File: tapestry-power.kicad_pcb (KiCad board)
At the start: 2 copper layers, 15 parts, among them J1 4.5-20V, J2 4.5-20V, J3 5V, U1 sic450

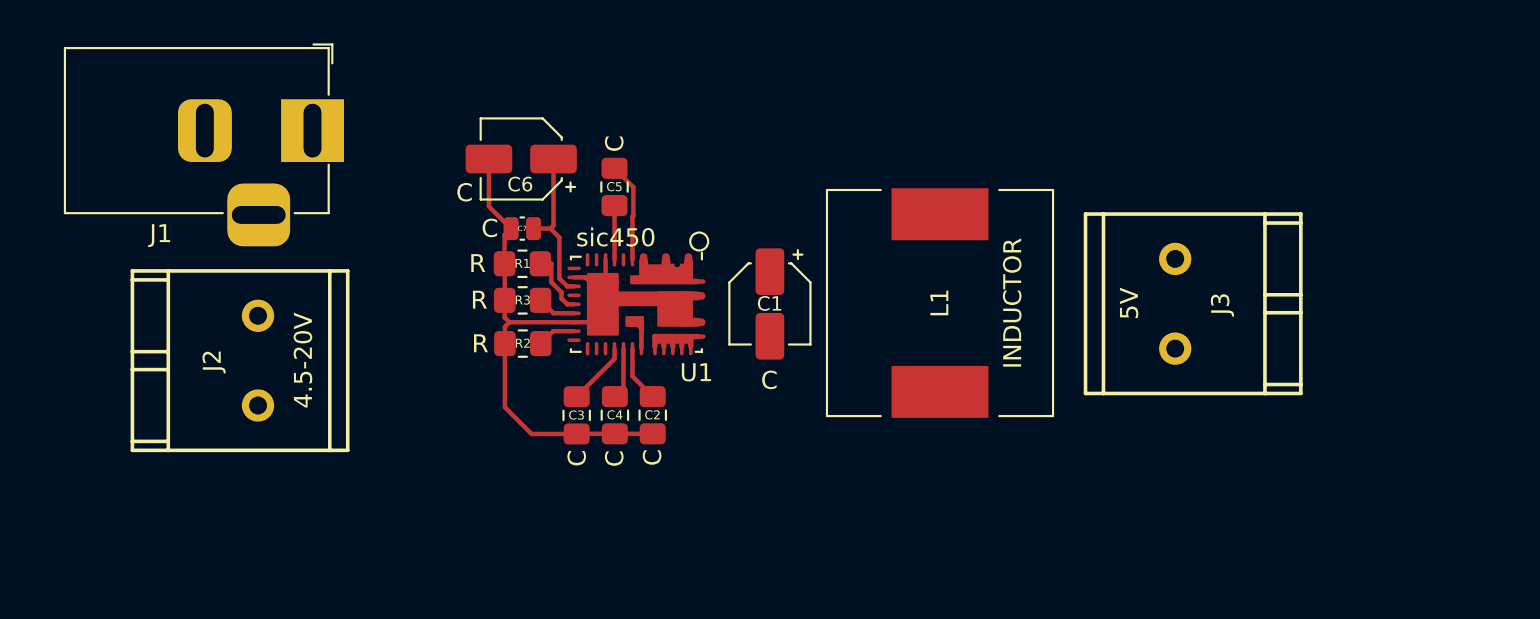
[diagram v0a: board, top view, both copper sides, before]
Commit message: basic board
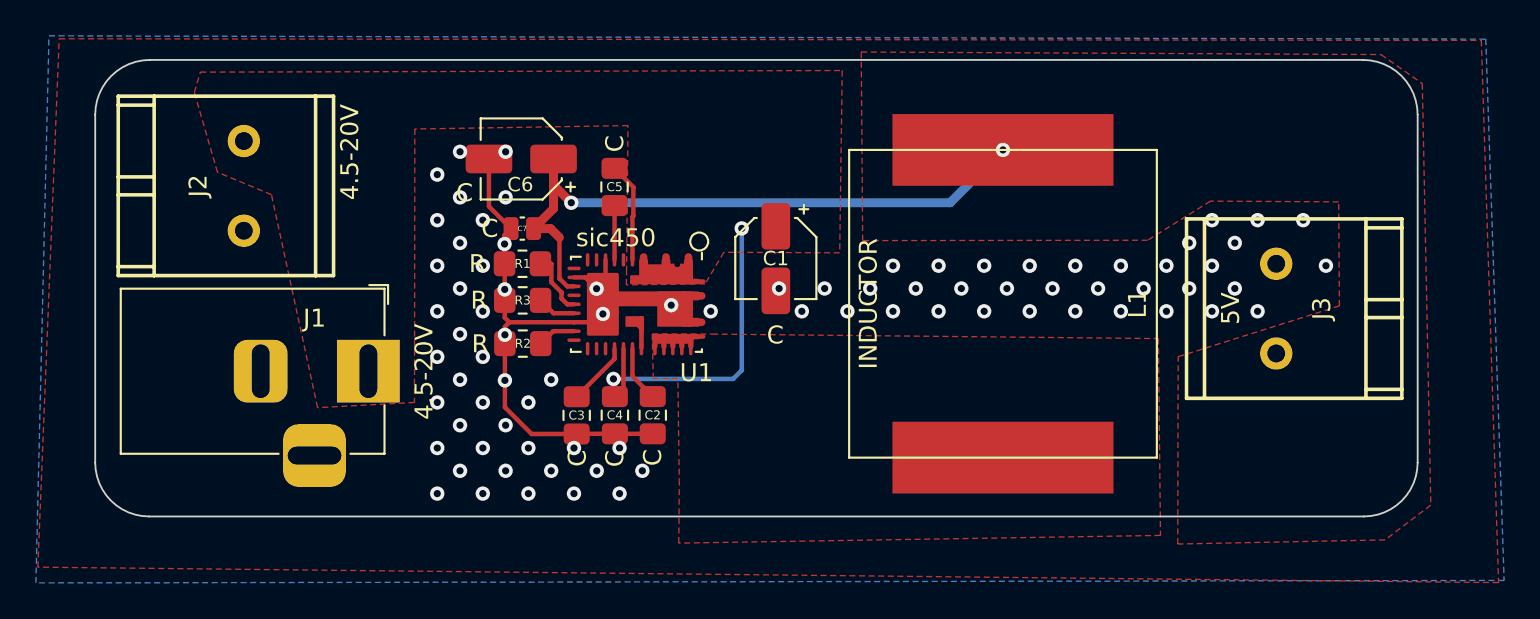
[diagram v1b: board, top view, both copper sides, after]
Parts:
- L1: footprint Inductor_SMD:L_12x12mm_H6mm -> libs:IP67GZ01
- moved J1 13.8 mm to (119.3, 68.1)
- moved J2 9.77 mm to (112.4, 55.3)
- moved J3 5.64 mm to (169.9, 67.1)
- moved L1 3.51 mm to (154.7, 64.3)
- moved C1 2.55 mm to (142.1, 61.8)
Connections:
- net Net-(L1-Pad1) renamed /VHIGH
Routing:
- net /VOUT: track 8.88 -> 38.1 mm, vias 0 -> 2
- net /VIN: track 5.38 -> 21.7 mm, vias 0 -> 2
- net GND: vias 0 -> 82
- added copper zone on F.Cu, net /VHIGH
- added copper zone on F.Cu, net /VIN
- added copper zone on F.Cu, net /VOUT
- added copper zone on B.Cu, net GND
- added copper zone on F.Cu, net GND
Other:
- board outline added: 73.7 x 25.4 mm
